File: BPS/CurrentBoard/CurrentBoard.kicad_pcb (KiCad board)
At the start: 2 copper layers, 30 parts, among them J1 ShuntConn, J2 LeaderConn, U1 AS8510-ASSM, U2 RO-123.3S_HP, U3 LTC6820, U4 HX1188FNL

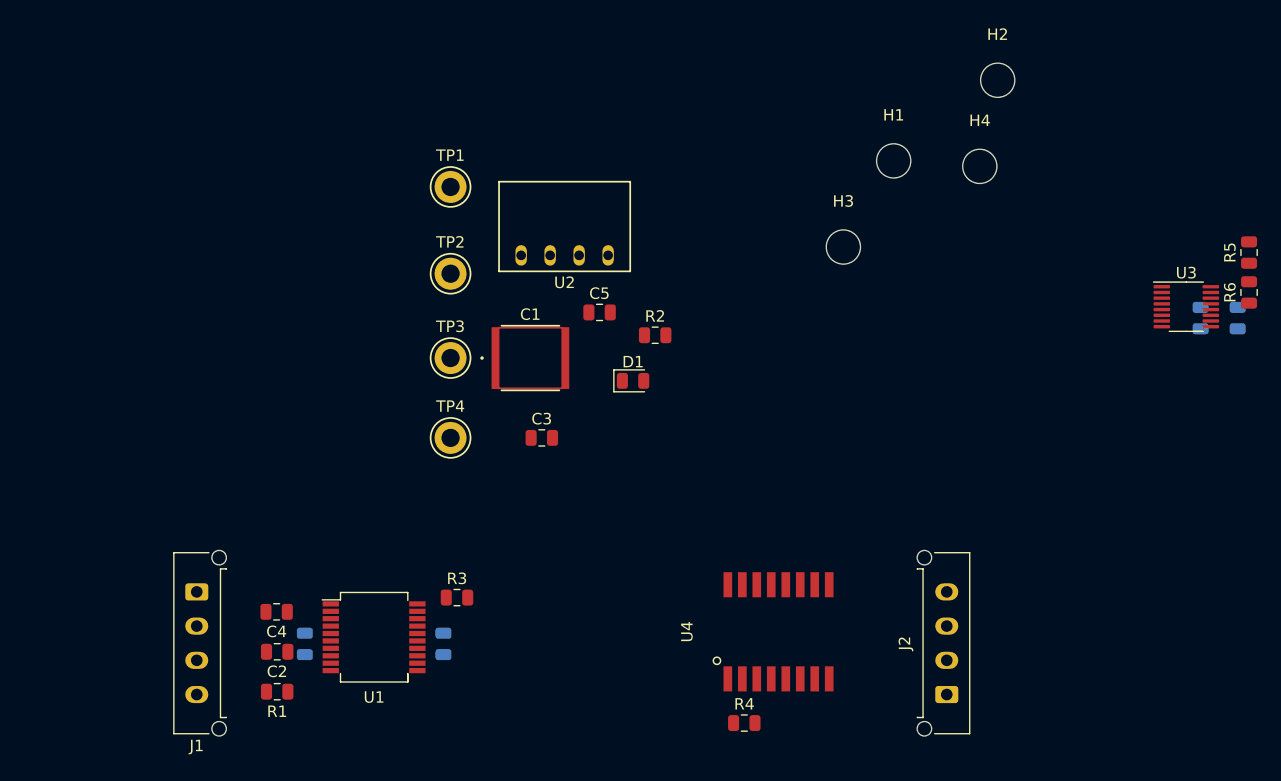
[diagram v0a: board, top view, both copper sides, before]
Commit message: Worked on layout of board
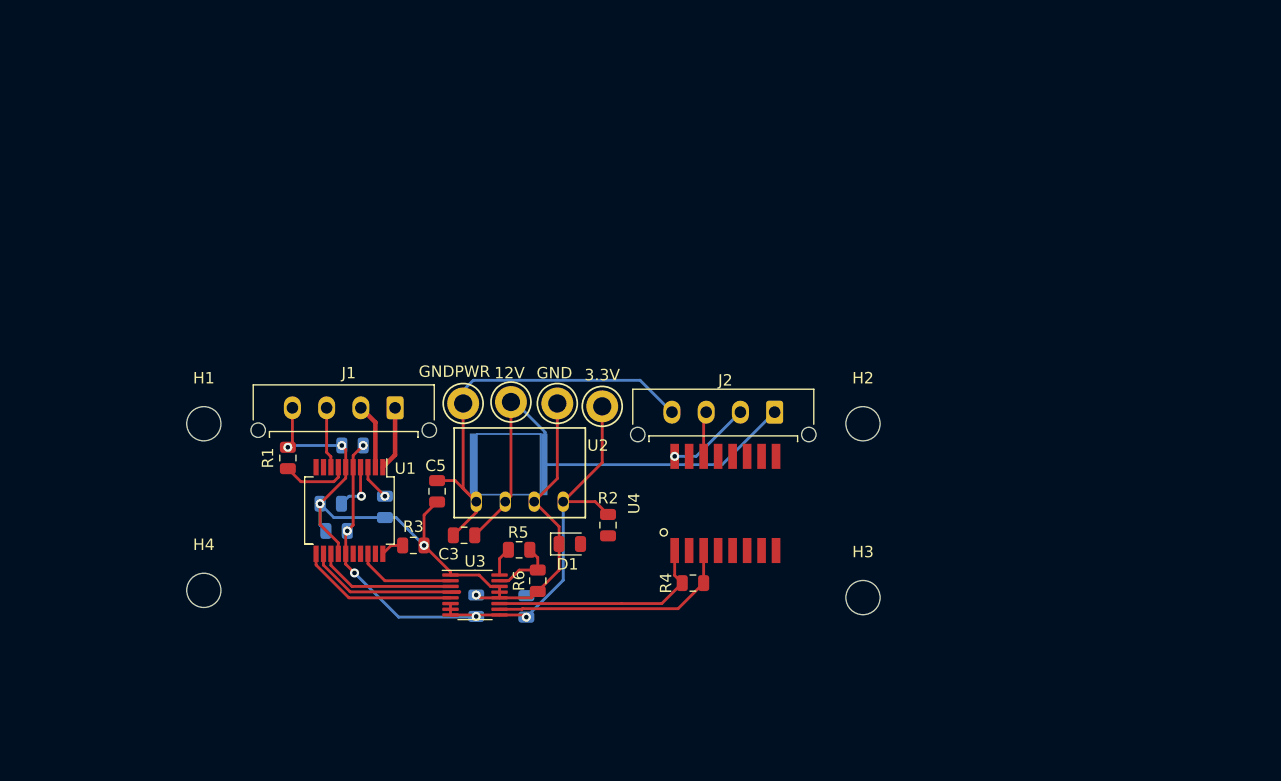
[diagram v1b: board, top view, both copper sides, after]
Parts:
- removed TP2: GNDPWR_TP, TestPoint:TestPoint_Keystone_5005-5009_Compact
- added GNDPWR: GNDPWR_TP, TestPoint:TestPoint_Keystone_5005-5009_Compact, F.Cu at (125.6, 110.0)
- C1, C2, C4: moved to B.Cu
- moved H4 77.5 mm to (102.9, 126.4)
- moved R5 69.1 mm to (130.5, 122.8), turned to 180 degrees
- moved C8 68.3 mm to (126.7, 127.7)
- moved C9 67.3 mm to (131.1, 127.8)
- moved R6 67.3 mm to (132.1, 125.5)
- moved U3 67.3 mm to (126.6, 126.8)
- moved H1 64.7 mm to (102.9, 111.8)
- moved H2 32.3 mm to (160.7, 111.8)
- moved H3 30.8 mm to (160.7, 127.0)
- moved J2 29.0 mm to (152.9, 110.7), turned to 180 degrees
- moved J1 23.7 mm to (119.6, 110.4), turned to 180 degrees
- moved U2 21.9 mm to (130.6, 118.6)
- moved C5 21.2 mm to (123.3, 117.7), turned to 270 degrees
- moved R1 20.5 mm to (110.2, 114.8), turned to 90 degrees
- moved 12V 19.6 mm to (129.8, 109.9)
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- renumbered TP1 to 12V, TP3 to 3.3V, TP4 to GND
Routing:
- net GND: track 0.00 -> 71.2 mm, vias 0 -> 5
- net +3V3: track 0.00 -> 57.9 mm, vias 0 -> 5
- net +12V: track 0.00 -> 42.0 mm
- net GNDPWR: track 0.00 -> 41.5 mm
- net /IM: track 0.00 -> 21.7 mm
- net /IP: track 0.00 -> 19.9 mm
- net /SCK: track 0.00 -> 14.7 mm
- net /CS: track 0.00 -> 14.0 mm
- net /MISO: track 0.00 -> 12.3 mm
- net /MOSI: track 0.00 -> 8.73 mm
- net Net-(J2-Pad2): track 0.00 -> 7.37 mm, vias 0 -> 1
- net Net-(R1-Pad1): track 0.00 -> 5.94 mm
- net Net-(R5-Pad1): track 0.00 -> 5.80 mm
- net /RSHL: track 0.00 -> 5.74 mm
- net /RSHH: track 0.00 -> 5.65 mm
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
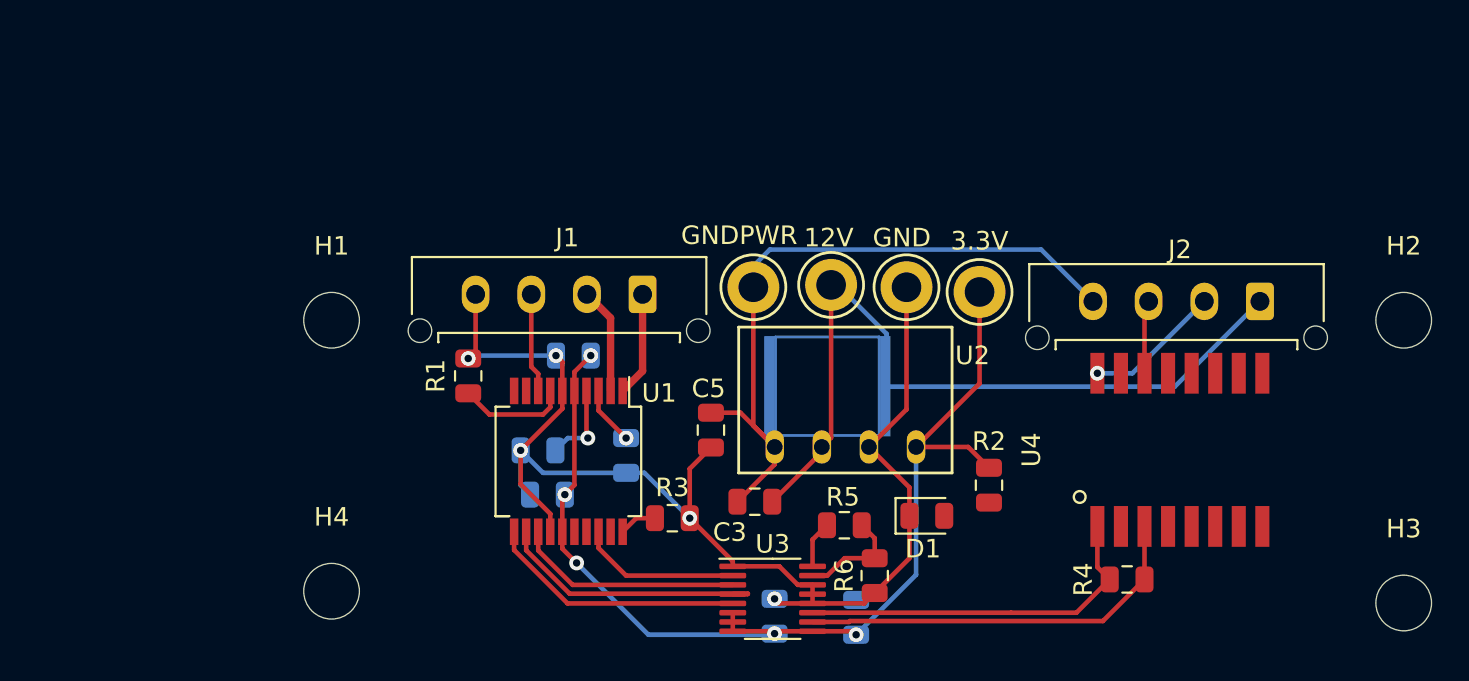
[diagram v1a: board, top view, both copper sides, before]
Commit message: Finishes PCB layout of current board
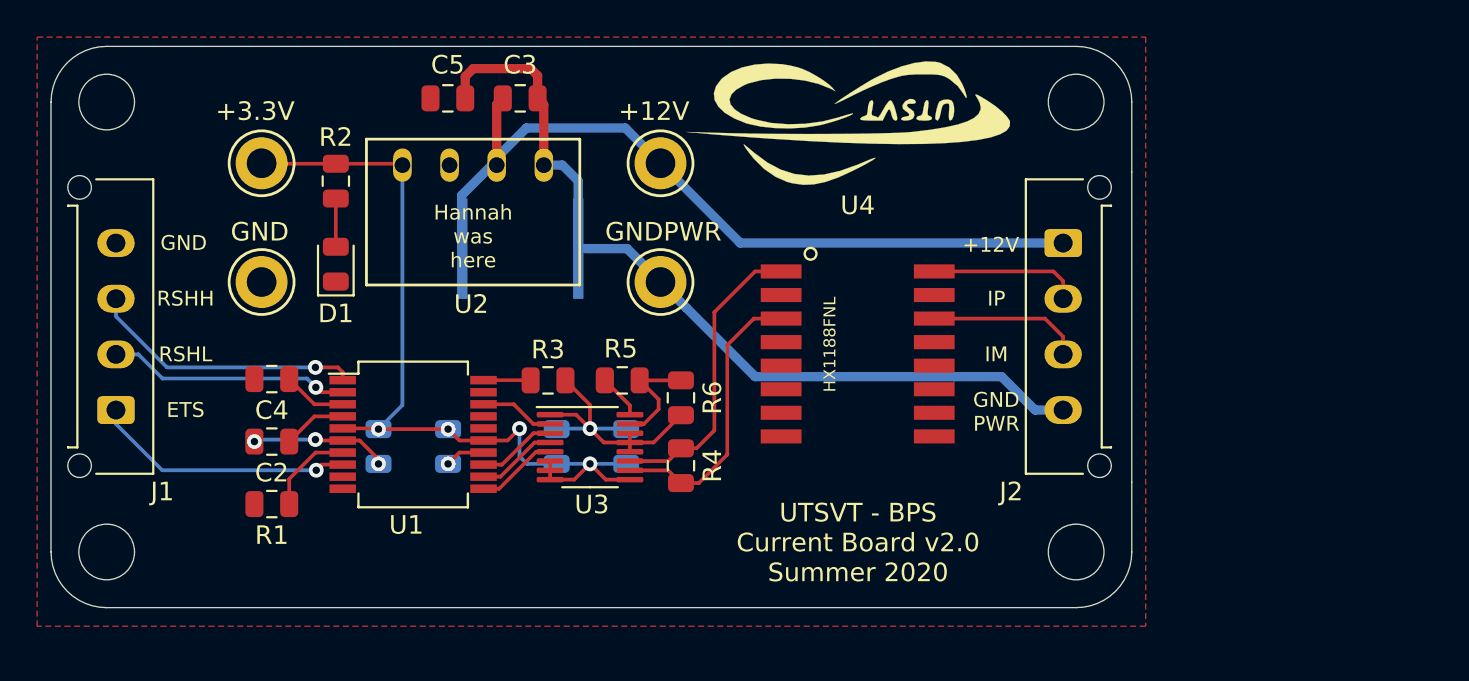
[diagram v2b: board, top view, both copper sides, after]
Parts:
- added G***: LOGO, UTSVT_Special:Hallock_Image_Tiny, B.Cu at (131.5, 116.2)
- added G***: LOGO, UTSVT_Special:UTSVT_Logo_Symbol, F.Cu at (131.0, 101.0)
- C2, C4: moved to F.Cu
- moved TP3 39.3 mm to (99.1, 103.3), turned to 90 degrees
- moved R2 38.8 mm to (103.1, 104.3)
- moved TP4 34.8 mm to (99.1, 109.7), turned to 90 degrees
- moved D1 34.6 mm to (103.1, 108.7), turned to 90 degrees
- moved J1 29.1 mm to (91.2, 116.6), turned to 90 degrees
- moved U2 25.2 mm to (110.5, 103.4), turned to 180 degrees
- moved C3 25.1 mm to (113.0, 99.8), turned to 0 degrees
- moved R4 24.8 mm to (121.7, 119.6), turned to 270 degrees
- moved C5 22.8 mm to (109.1, 99.8), turned to 180 degrees
- moved H2 21.2 mm to (143.0, 100.0)
- moved C4 19.5 mm to (99.7, 114.9), turned to 0 degrees
- moved C1 18.1 mm to (113.0, 107.9), turned to 0 degrees
- moved U4 18.1 mm to (131.2, 113.6), turned to 270 degrees
- moved H3 17.9 mm to (143.0, 124.2)
- moved H1 16.9 mm to (90.8, 100.0)
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- renumbered 12V to TP1, GNDPWR to TP2, 3.3V to TP3, GND to TP4
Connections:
- J1 pad 1: /RSHH -> /ETS
- J1 pad 3: /ETS -> /RSHH
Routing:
- net GND: track 71.2 -> 25.8 mm
- net +3V3: track 57.9 -> 45.9 mm, vias 5 -> 4
- net /SCK: track 14.7 -> 4.35 mm
- net /CS: track 14.0 -> 4.41 mm
- net /RSHH: track 5.65 -> 14.8 mm, vias 0 -> 1
- net /ETS: track 5.36 -> 14.1 mm, vias 0 -> 1
- net /MISO: track 12.3 -> 4.29 mm
- net /RSHL: track 5.74 -> 13.1 mm, vias 0 -> 1
- net /IM: track 21.7 -> 15.6 mm
- net /MOSI: track 8.73 -> 4.03 mm
- net Net-(J2-Pad3): track 3.97 -> 8.30 mm
- net GNDPWR: track 41.5 -> 45.6 mm
- net /IP: track 19.9 -> 16.1 mm
- net Net-(D1-Pad2): track 0.00 -> 2.60 mm
- net +12V: track 42.0 -> 43.3 mm
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- added copper zone on F.Cu, net GND
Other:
- board outline added: 58.2 x 30.2 mm
- net class Default: clearance 0.2 -> 0.127
- rule trace_clearance: 0.2 -> 0.127
- board text added: "+12V"
- board text added: "+3.3V"
- board text added: "Dr. Gary Hallock"
- board text added: "ETS"
- board text added: "GND"
- board text added: "GND PWR"
- board text added: "GNDPWR"
- board text added: "Hannah was here"
- board text added: "IM"
- board text added: "IP"
- board text added: "RSHH"
- board text added: "RSHL"
- board text added: "UTSVT - BPS Current Board v2.0 Summer 2020"
